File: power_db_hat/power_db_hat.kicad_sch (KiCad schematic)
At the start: 32 parts, among them J2 BAT2, J5 24V_out, J8 BAT1, U7 B2B pins

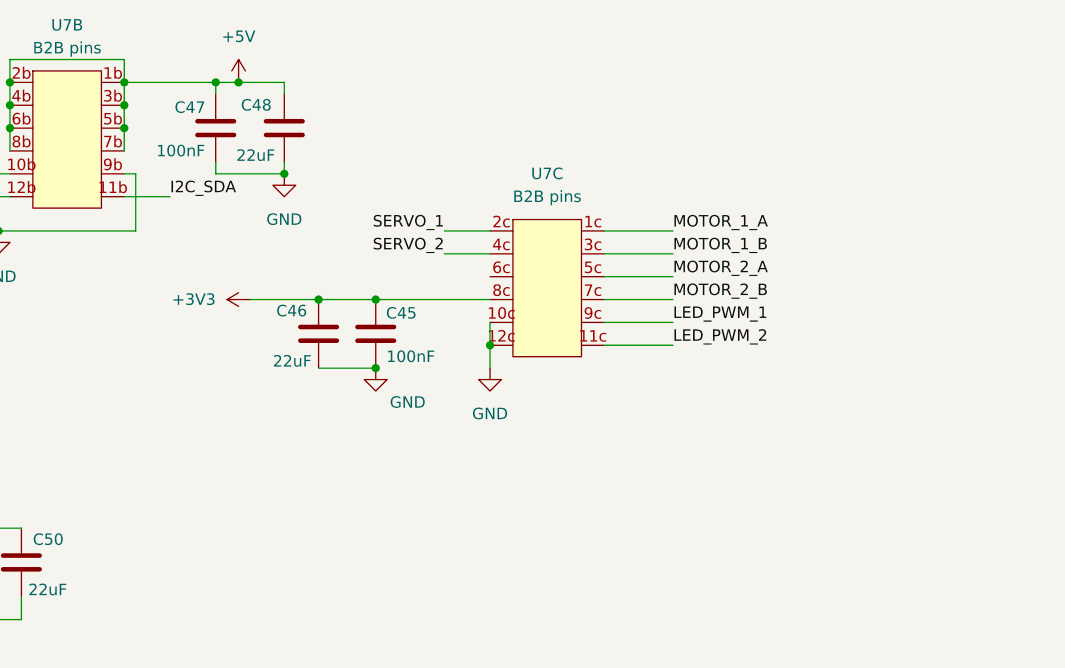
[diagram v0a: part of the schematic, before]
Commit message: lol
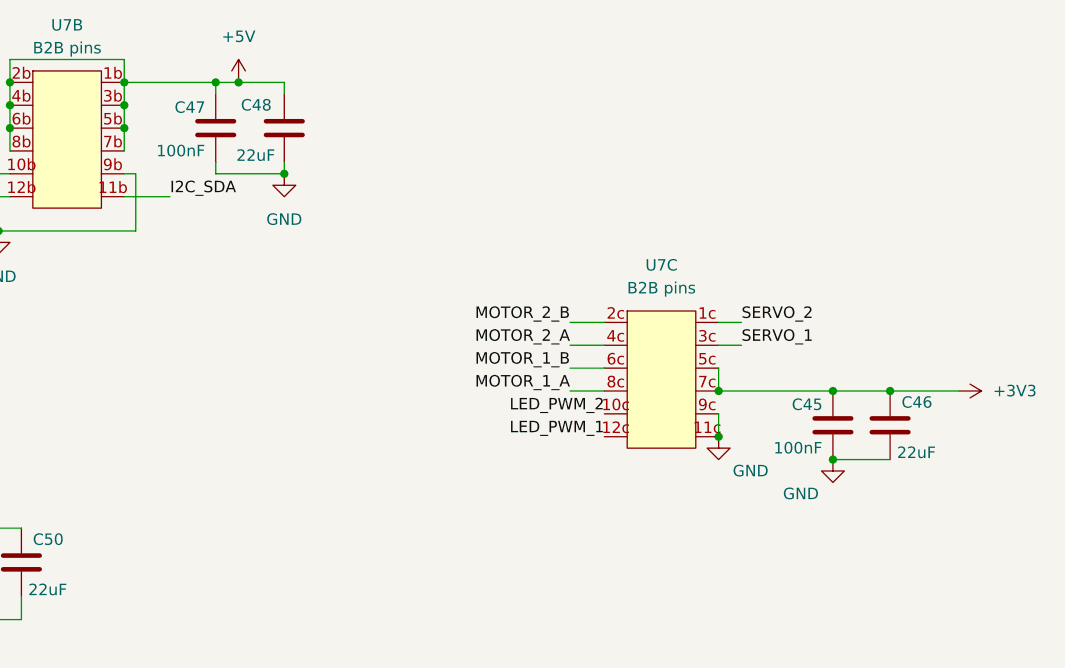
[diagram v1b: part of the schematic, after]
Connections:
- net +3V3: now also U7.5c, U7.7c; no longer U7.8c
- net GND: now also U7.11c, U7.9c; no longer U7.10c, U7.12c
- net LED_PWM_1: now also U7.12c; no longer U7.9c
- net LED_PWM_2: now also U7.10c; no longer U7.11c
- net MOTOR_1_A: now also U7.8c; no longer U7.1c
- net MOTOR_1_B: now also U7.6c; no longer U7.3c
- net MOTOR_2_A: now also U7.4c; no longer U7.5c
- net MOTOR_2_B: now also U7.2c; no longer U7.7c
- net SERVO_1: now also U7.3c; no longer U7.2c
- net SERVO_2: now also U7.1c; no longer U7.4c
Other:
- moved on the sheet: C45, C46, U7C
